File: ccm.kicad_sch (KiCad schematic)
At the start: 40 parts, among them J1 Conn_01x02_Socket, J2 Conn_01x02_Socket, J3 Conn_01x02_Socket, J4 Conn_01x04_Socket, J6 Conn_01x02_Socket, J7 Conn_01x02_Socket, J8 Conn_01x04_Socket, J9 Conn_01x02_Socket, Q1 IRLZ34N, U1 Teensy4.1, U2 PAM8302AAY, U3 SN65HVD230, U4 SN65HVD230, U5 LM1117DT-5.0

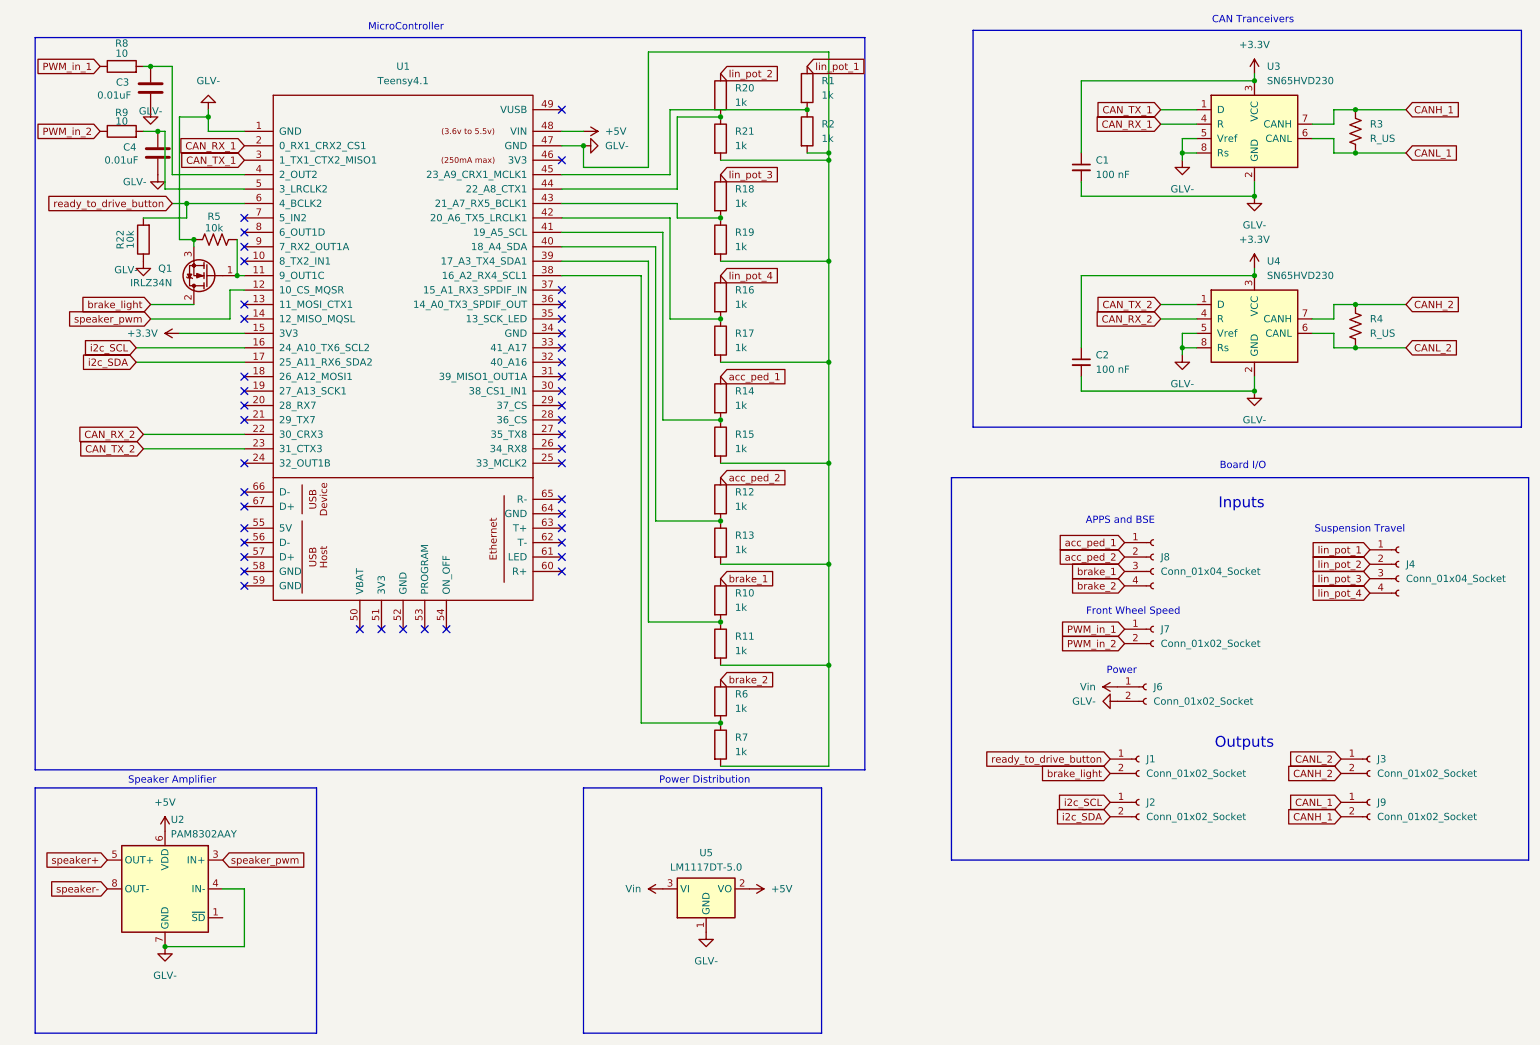
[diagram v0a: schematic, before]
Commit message: right side routed
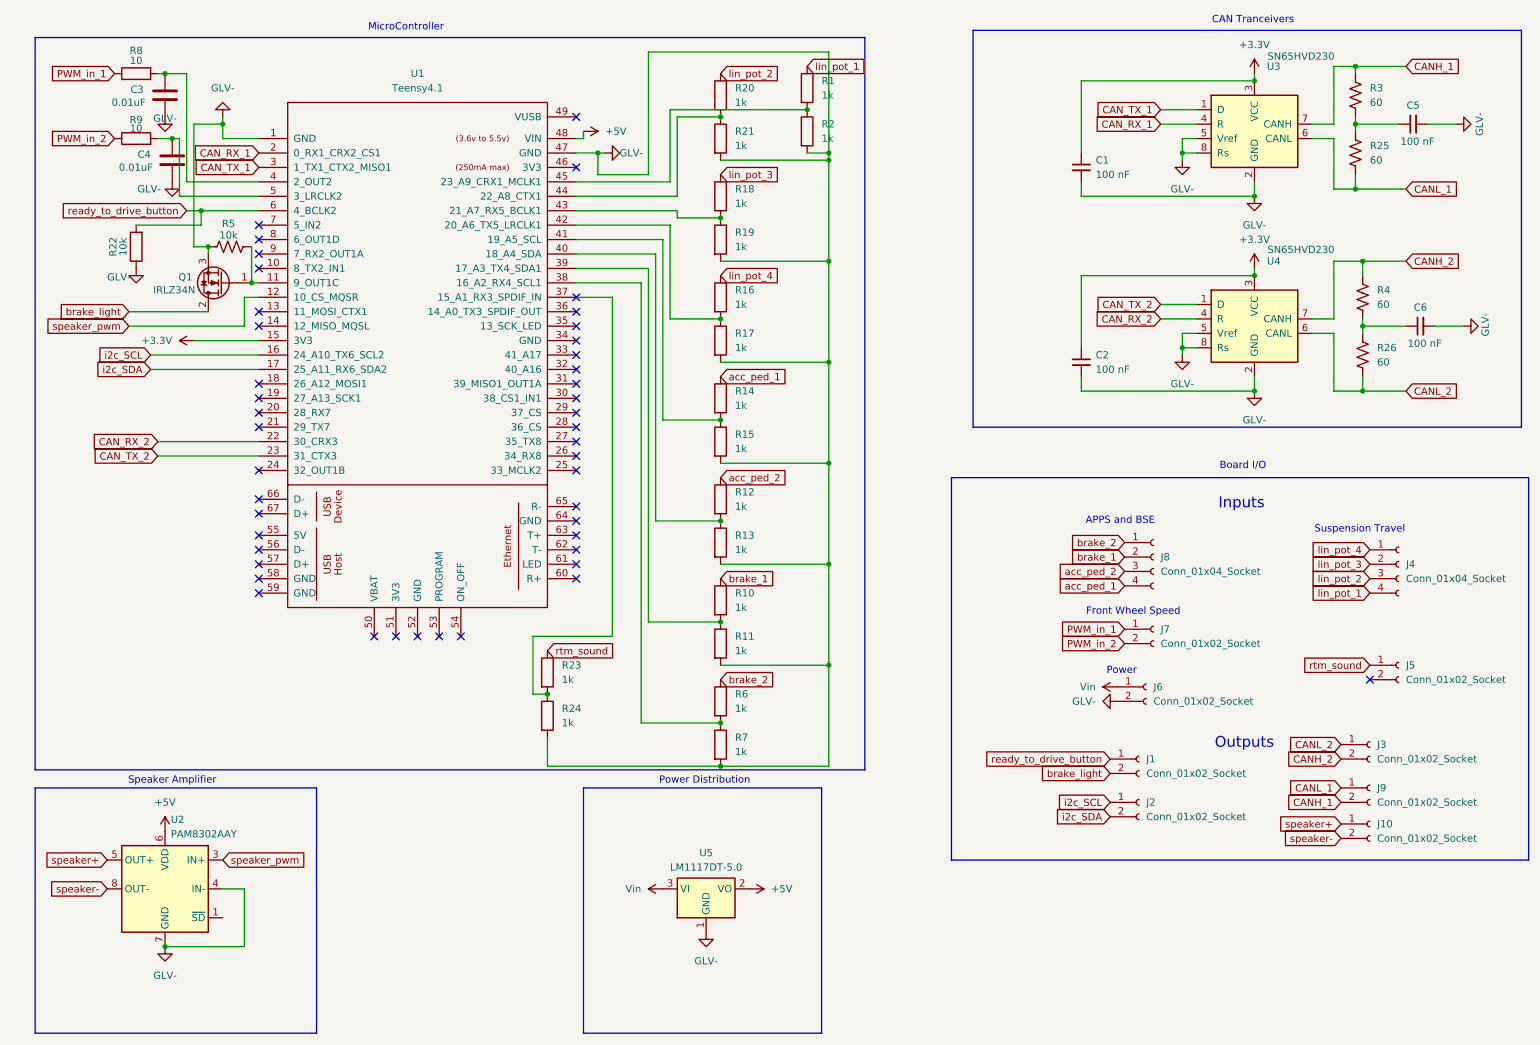
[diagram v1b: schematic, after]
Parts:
- added C5, C6: 100 nF, Capacitor_SMD:C_0805_2012Metric, symbol Device:C_Small
- added J10, J5: Conn_01x02_Socket, Connector_Molex:Molex_Mini-Fit_Jr_5566-02A2_2x01_P4.20mm_Vertical, symbol Connector:Conn_01x02_Socket
- added R23, R24: 1k, Resistor_SMD:R_0805_2012Metric, symbol Device:R
- added R25, R26: 60, Resistor_SMD:R_0805_2012Metric, symbol Device:R_US
- R3, R4: value R_US -> 60
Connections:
- net CANL_1: now also R25.2; no longer R3.2
- net CANL_2: now also R26.2; no longer R4.2
- net GLV-: now also C5.2, C6.2, R24.2
- net acc_ped_1: now also J8.4 (Pin_4); no longer J8.1 (Pin_1)
- net acc_ped_2: now also J8.3 (Pin_3); no longer J8.2 (Pin_2)
- net brake_1: now also J8.2 (Pin_2); no longer J8.3 (Pin_3)
- net brake_2: now also J8.1 (Pin_1); no longer J8.4 (Pin_4)
- net lin_pot_1: now also J4.4 (Pin_4); no longer J4.1 (Pin_1)
- net lin_pot_2: now also J4.3 (Pin_3); no longer J4.2 (Pin_2)
- net lin_pot_3: now also J4.2 (Pin_2); no longer J4.3 (Pin_3)
- net lin_pot_4: now also J4.1 (Pin_1); no longer J4.4 (Pin_4)
- net speaker+: now also J10.1 (Pin_1)
- net speaker-: now also J10.2 (Pin_2)
- net at U1.37 (15_A1_RX3_SPDIF_IN): now also R23.2, R24.1
- new net: C6.1, R26.1, R4.2
- new net: C5.1, R25.1, R3.2
- new net rtm_sound: J5.1 (Pin_1), R23.1
- no-connect marks 44 -> 45
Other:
- moved on the sheet: C3, C4, J3, J9, Q1, R22, R3, R5, R8, R9, U1
